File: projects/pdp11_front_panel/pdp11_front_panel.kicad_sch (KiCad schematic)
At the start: 0 parts

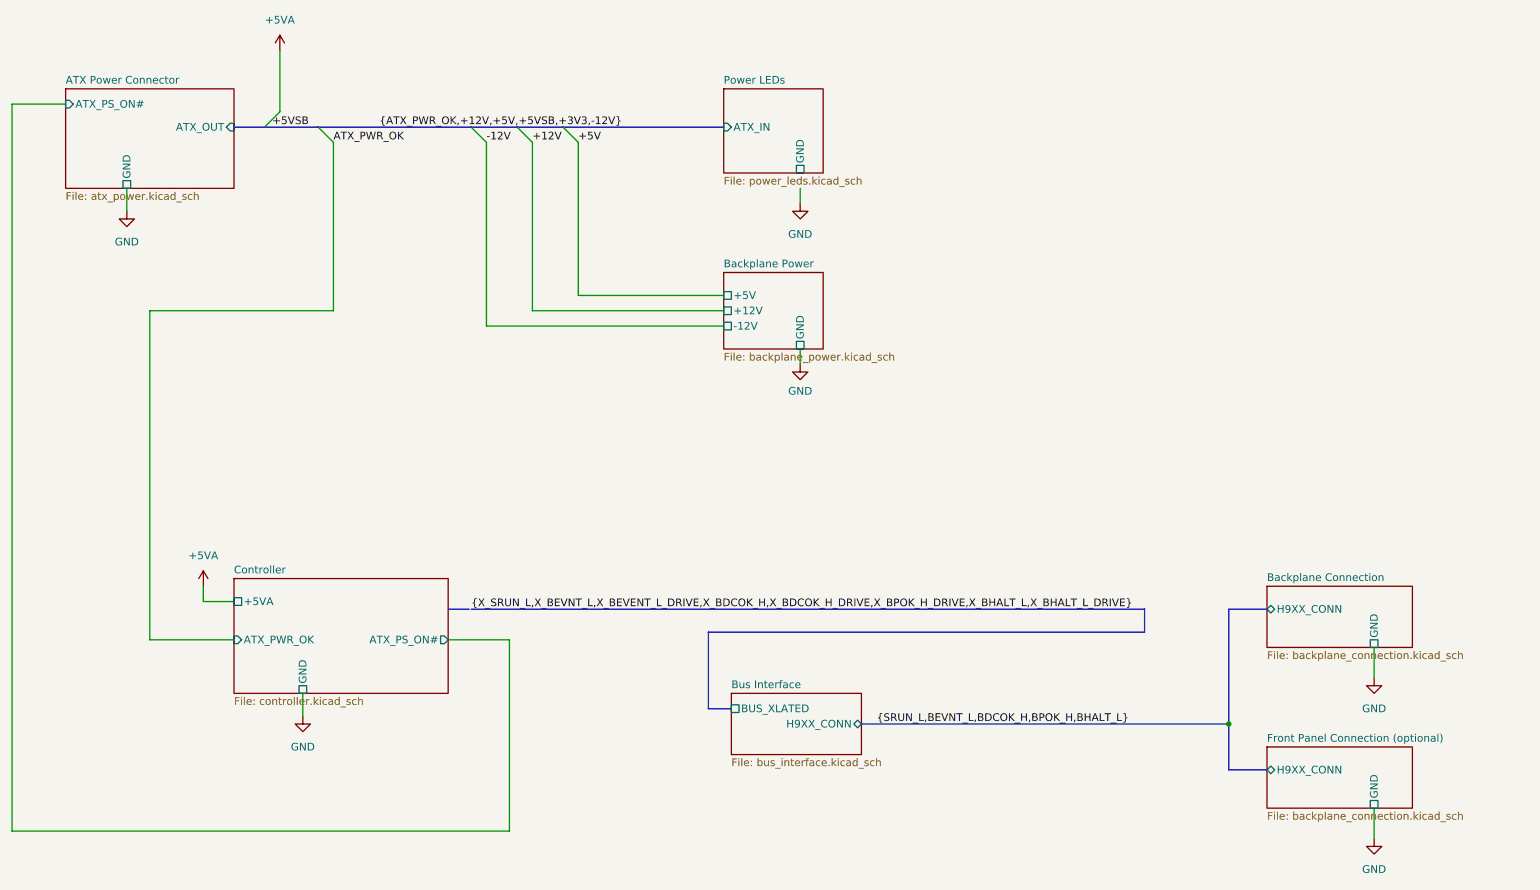
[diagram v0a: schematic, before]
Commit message: wip
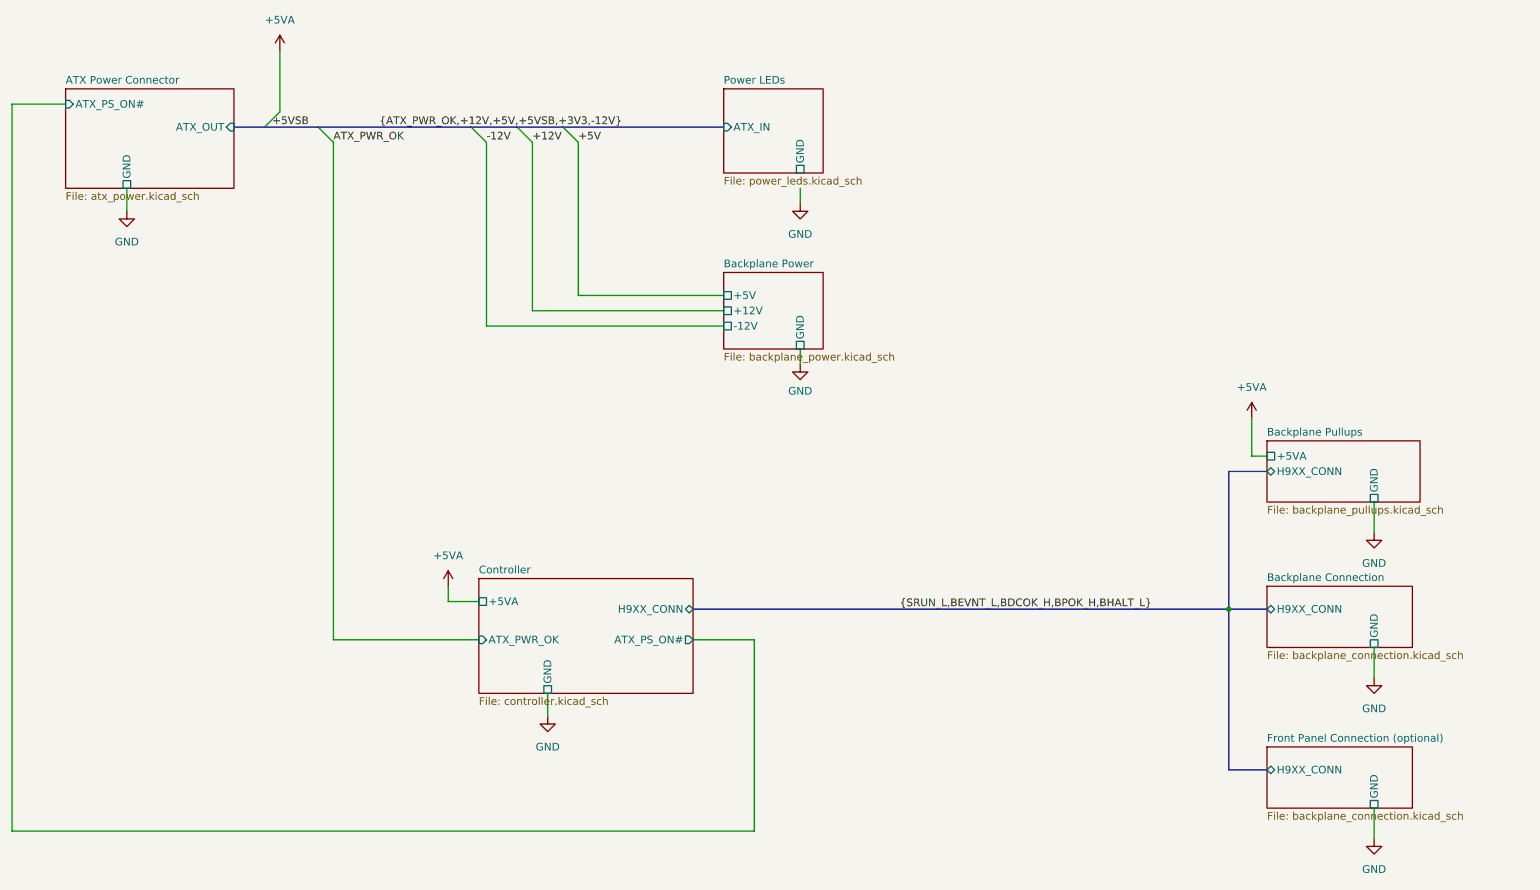
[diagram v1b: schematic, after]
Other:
- removed sheet Bus Interface
- added sheet Backplane Pullups (backplane_pullups.kicad_sch)
- sheet Controller ports: added H9XX_CONN; removed none
